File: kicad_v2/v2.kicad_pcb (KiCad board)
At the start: 2 copper layers, 106 parts, among them P1 ESP_RX_TX, P10 LED_conf1, P11 LED_conf2, P12 CONN_01X01, P13 CONN_01X01, P14 CONN_01X01, P15 CONN_01X01, P2 CON_MEANWELL_VDC, P3 CON_LED1, P4 CON_DIM, P5 CON_DS18B20, P6 CON_230V, P7 CON_MEANWELL, P8 CONN_01X02, P9 CON_LED2, Q1 bc847, Q2 bc847, U1 LD1117S33TR, U2 LD1117S33TR, U3 mini_ESP8266, U4 MCP6V31, U5 MCP3208, U6 LM358, U7 LM393, U8 MCP47X6

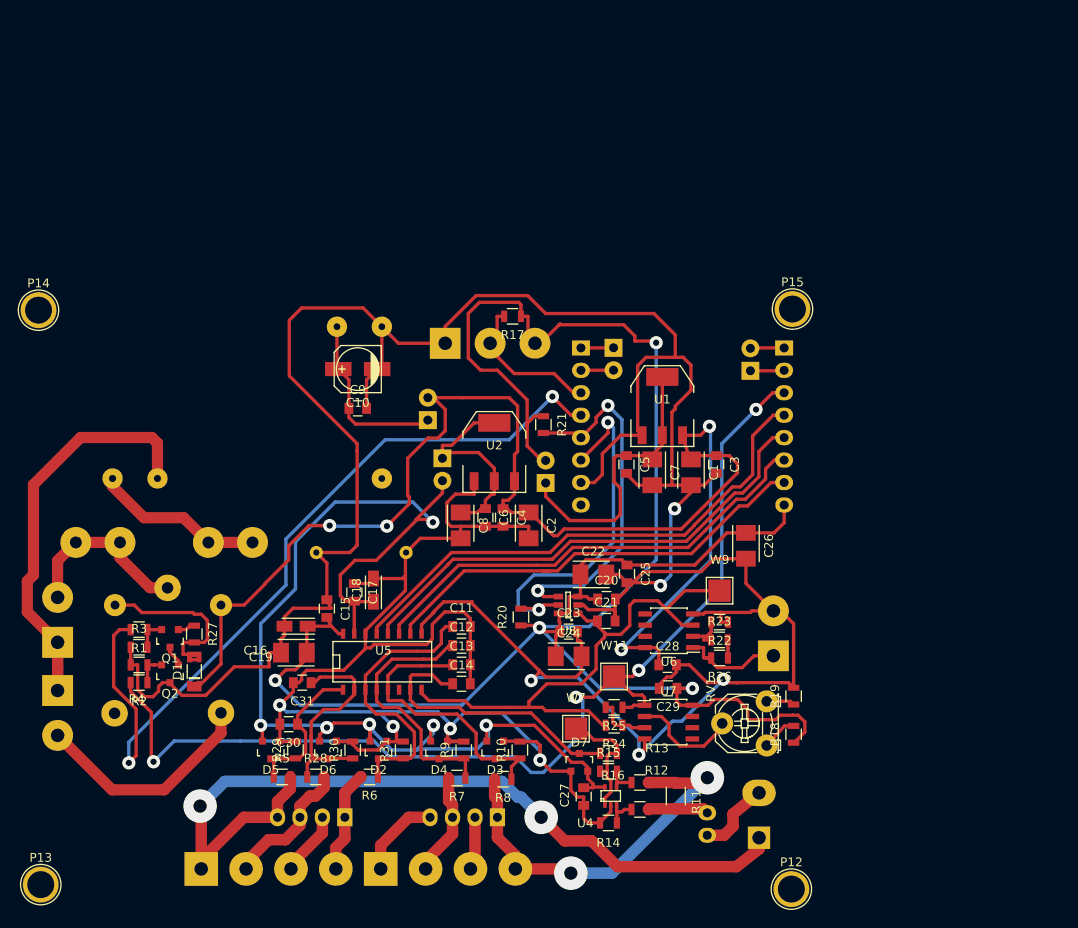
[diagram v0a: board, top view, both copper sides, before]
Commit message: new version
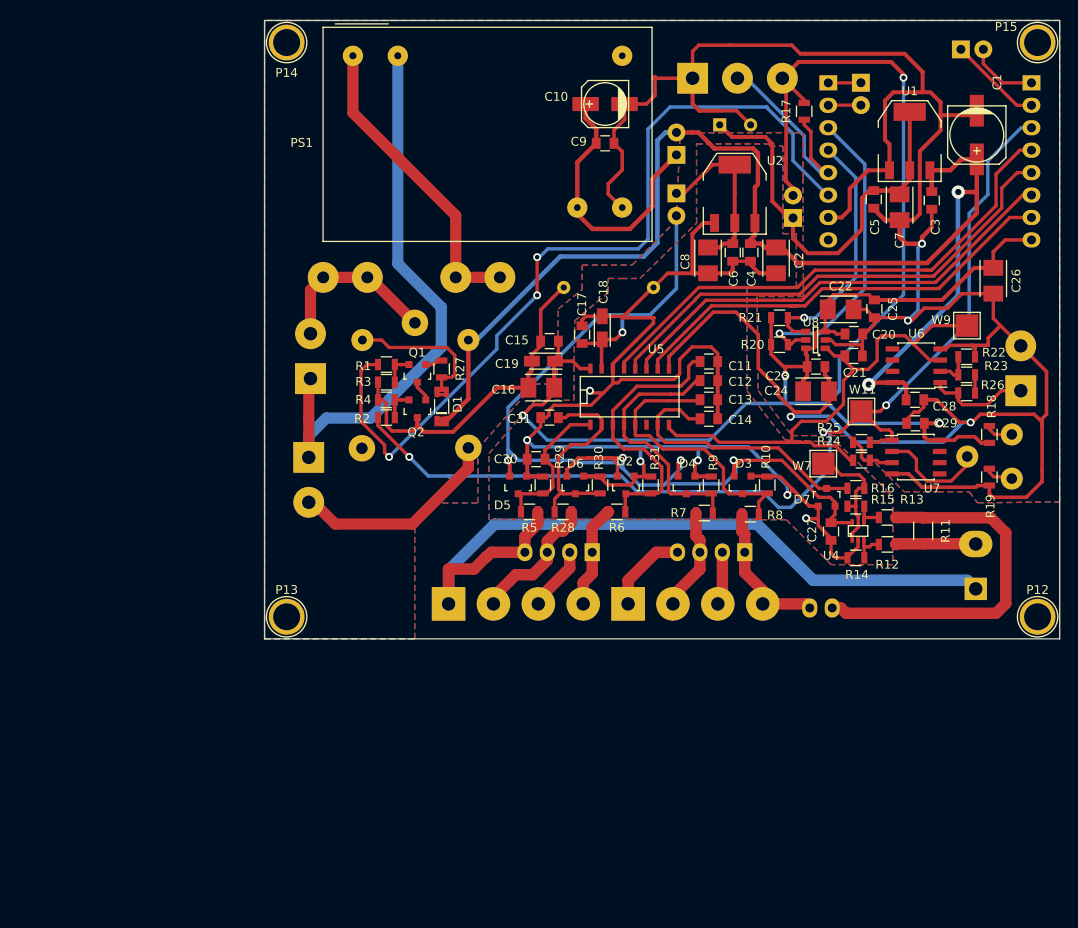
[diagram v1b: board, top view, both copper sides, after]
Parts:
- added C32: 470u, Capacitors_ThroughHole:C_Radial_D8_L11.5_P3.5, B.Cu at (154.4, 69.5)
- C1: value 10u -> 100u; footprint Capacitors_Tantalum_SMD:TantalC_SizeB_EIA-3528_Reflow -> Capacitors_SMD:c_elec_6.3x5.3
- PS1: moved to F.Cu
- RV1: moved to B.Cu
- moved PS1 55.0 mm to (112.9, 61.6)
- moved C1 50.0 mm to (183.6, 70.6)
- moved RV1 44.8 mm to (187.5, 104.5), turned to 270 degrees
- moved P8 43.5 mm to (181.8, 60.9), turned to 270 degrees
- moved R20 42.5 mm to (161.2, 94.3), turned to 0 degrees
- moved P12 41.6 mm to (190.4, 125.1)
- moved P6 41.4 mm to (108.1, 95.6)
- moved P14 41.3 mm to (105.4, 60.1)
- moved P13 41.2 mm to (105.4, 125.1)
- moved JP4 41.1 mm to (149.6, 72.8)
- moved R22 41.0 mm to (182.4, 95.7)
- moved C13 41.0 mm to (153.2, 100.6)
- moved C11 41.0 mm to (153.2, 96.2)
- moved C14 41.0 mm to (153.2, 102.7)
- moved C27 41.0 mm to (167.1, 115.5)
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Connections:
- JP1 pad 1: LED_Current_meas_in -> Net-(JP1-Pad1)
- JP1 pad 2: Net-(JP1-Pad2) -> LED1+
- R11 pad 1: Net-(JP1-Pad2) -> LED_Current_meas_in
- R11 pad 2: LED1+ -> Net-(JP1-Pad1)
- R12 pad 2: Net-(JP1-Pad2) -> LED_Current_meas_in
- R13 pad 2: LED1+ -> Net-(JP1-Pad1)
- U3 pad 11: DAC_SCL -> LED_ON
- U3 pad 12: DAC_SDA -> DS18B20
- U3 pad 13: LED_ON -> DAC_SDA
- U3 pad 14: DS18B20 -> DAC_SCL
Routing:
- net Net-(JP1-Pad1): track 0.00 -> 41.5 mm
- net LED1+: track 44.5 -> 16.6 mm, vias 2 -> 0
- net +3V3: track 233.9 -> 210.6 mm
- net Net-(F1-Pad2): track 20.0 -> 35.6 mm
- net Net-(C32-Pad1): track 32.5 -> 47.7 mm
- net AC_N: track 50.7 -> 65.8 mm
- net +3.3VADC: track 132.9 -> 119.5 mm, vias 6 -> 5
- net DAC_SDA: track 40.2 -> 28.5 mm, vias 2 -> 1
- net Net-(C10-Pad1): track 20.3 -> 31.9 mm
- net DS18B20: track 17.2 -> 28.3 mm
- net Net-(P8-Pad1): track 3.84 -> 11.3 mm
- net GND: track 348.3 -> 341.1 mm, vias 5 -> 4
- net Net-(JP1-Pad2): track 6.89 -> 0.00 mm
- net LED4-: track 94.4 -> 88.3 mm, vias 2 -> 0
- net GNDA: track 160.7 -> 166.3 mm, vias 4 -> 6
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- added copper zone on B.Cu, net GND
- added copper zone on F.Cu, net GND
- added copper zone on B.Cu, net GNDA
- added copper zone on F.Cu, net GNDA
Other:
- board outline added: 90 x 70 mm
- net class 12V added: clearance 0.254, trace_width 0.508, via_dia 1.5, via_drill 0.7
- net class Default: via_dia 1.5 -> 0.9; via_drill 0.7 -> 0.5
- net class power_LV added: clearance 0.254, trace_width 0.4064, via_dia 0.9, via_drill 0.5
